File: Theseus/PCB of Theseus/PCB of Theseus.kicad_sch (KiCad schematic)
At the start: 47 parts, among them J1 Screw_Terminal_01x04, J2 Screw_Terminal_01x04, J4 Screw_Terminal_01x06, J7 Screw_Terminal_01x02, J8 Screw_Terminal_01x06, Q1 NMOS, Q2 NMOS, U1 TPS564257DRL, U2 MCP2562

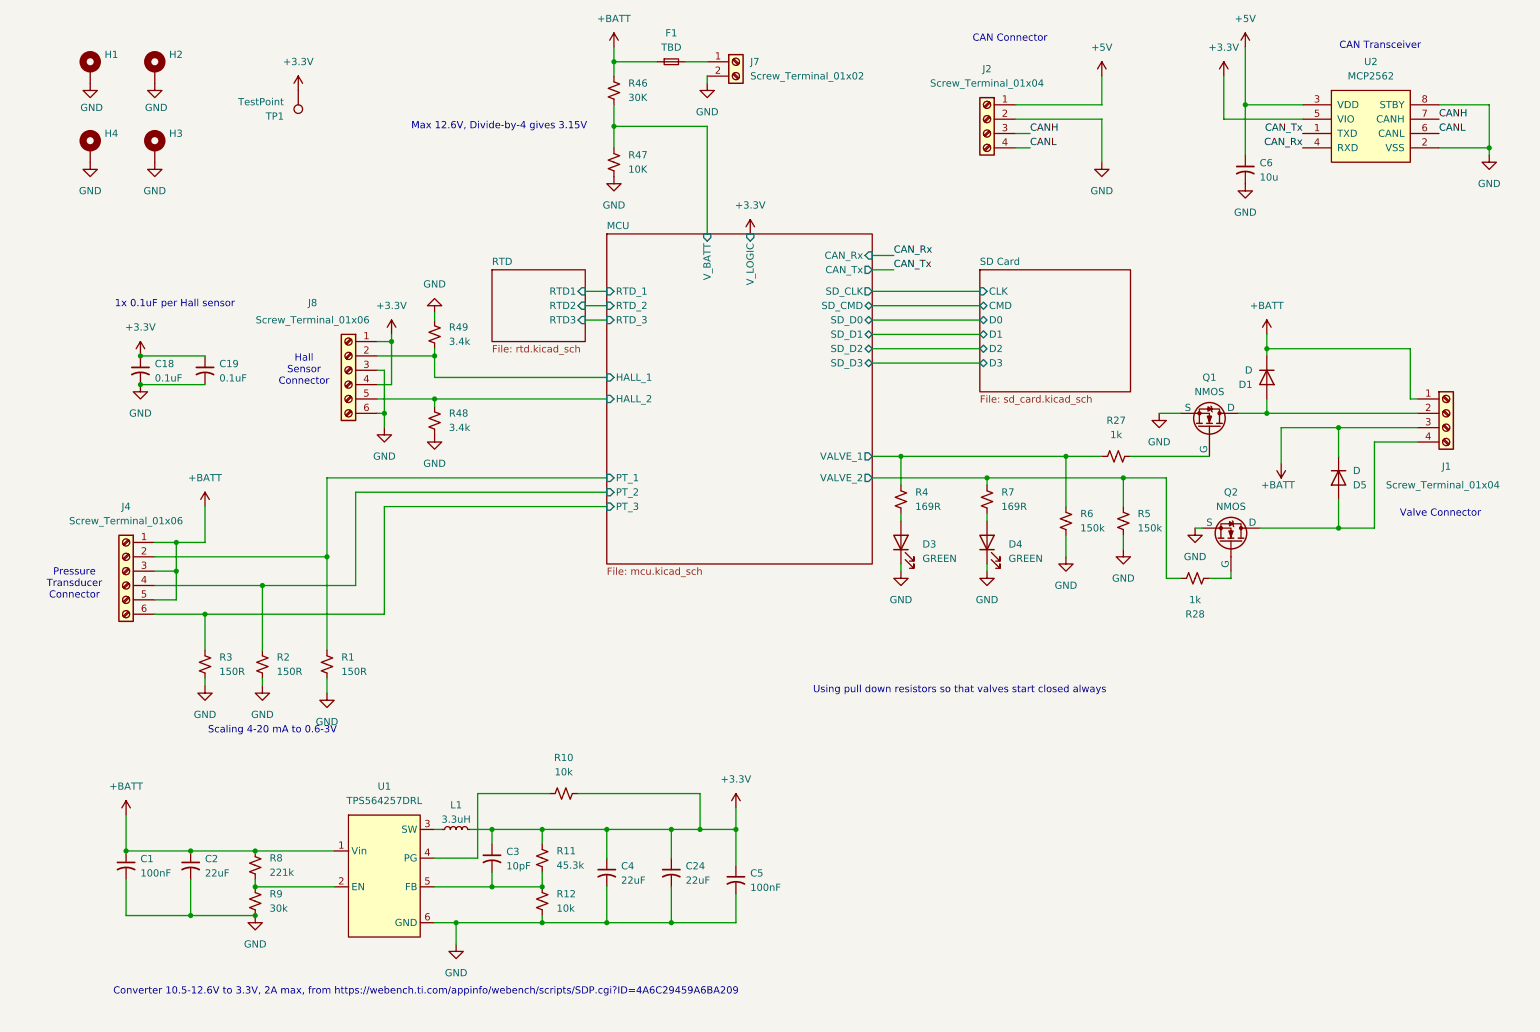
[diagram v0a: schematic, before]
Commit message: Theseus_Dev_Rev2
It's still the same PCB
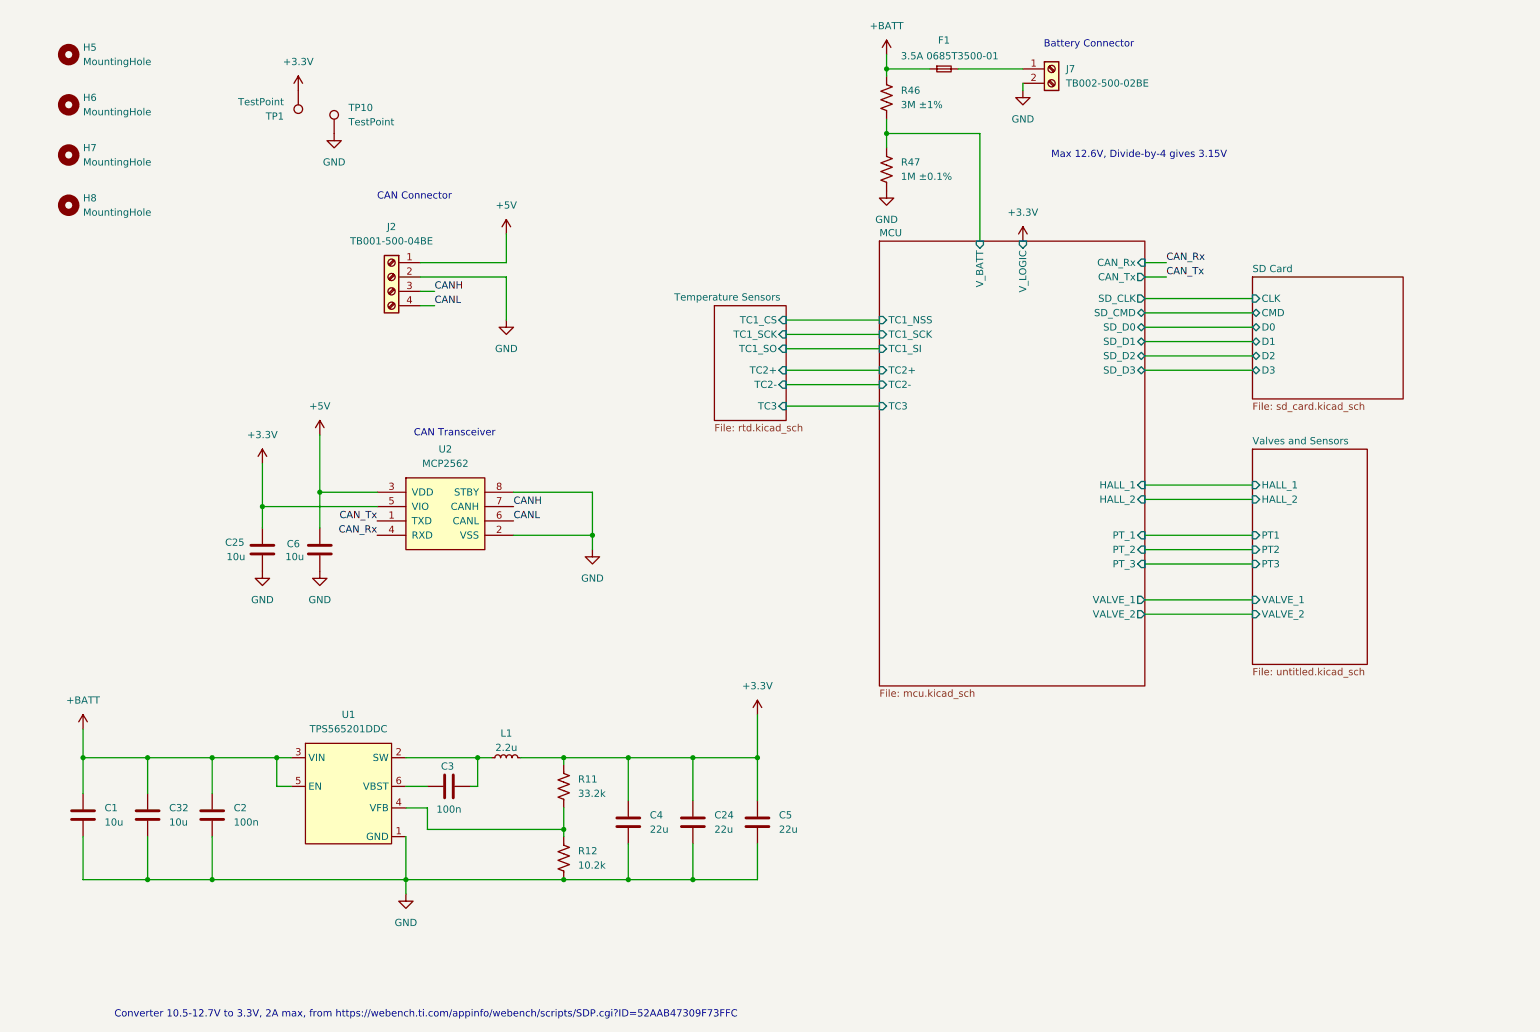
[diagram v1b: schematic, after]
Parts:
- removed C1, C5: 100nF, Capacitor_SMD:C_0603_1608Metric_Pad1.08x0.95mm_HandSolder, symbol Device:C_Small_US
- removed C18, C19: 0.1uF, Capacitor_SMD:C_0201_0603Metric_Pad0.64x0.40mm_HandSolder, symbol Device:C_Small_US
- removed C2, C24, C4: 22uF, Capacitor_SMD:C_0805_2012Metric_Pad1.18x1.45mm_HandSolder, symbol Device:C_Small_US
- removed C3: 10pF, Capacitor_SMD:C_0402_1005Metric_Pad0.74x0.62mm_HandSolder, symbol Device:C_Small_US
- removed C6: 10u, Capacitor_SMD:C_0603_1608Metric_Pad1.08x0.95mm_HandSolder, symbol Device:C_Small_US
- removed D1, D5: D, Diode_SMD:D_SMB-SMC_Universal_Handsoldering, symbol Device:D
- removed D3, D4: GREEN, Diode_SMD:D_0603_1608Metric_Pad1.05x0.95mm_HandSolder, symbol Device:LED
- removed H1, H2, H3, H4: ~, MountingHole:MountingHole_3.2mm_M3_Pad_Via, symbol Mechanical:MountingHole_Pad
- removed J1: Screw_Terminal_01x04, TerminalBlock_CUI:TerminalBlock_CUI_TB007-508-04_1x04_P5.08mm_Horizontal, symbol Connector:Screw_Terminal_01x04
- removed J4, J8: Screw_Terminal_01x06, TerminalBlock_CUI:TerminalBlock_CUI_TB007-508-06_1x06_P5.08mm_Horizontal, symbol Connector:Screw_Terminal_01x06
- removed Q1, Q2: NMOS, Package_TO_SOT_SMD:SOT-23-3, symbol Simulation_SPICE:NMOS
- removed R1, R2, R3: 150R, Resistor_SMD:R_0603_1608Metric_Pad0.98x0.95mm_HandSolder, symbol Device:R_Small_US
- removed R10: 10k, Resistor_SMD:R_0402_1005Metric_Pad0.72x0.64mm_HandSolder, symbol Device:R_Small_US
- removed R27, R28: 1k, Resistor_SMD:R_0402_1005Metric_Pad0.72x0.64mm_HandSolder, symbol Device:R_Small_US
- removed R4, R7: 169R, Resistor_SMD:R_0603_1608Metric_Pad0.98x0.95mm_HandSolder, symbol Device:R_Small_US
- removed R48, R49: 3.4k, Resistor_SMD:R_0402_1005Metric_Pad0.72x0.64mm_HandSolder, symbol Device:R_Small_US
- removed R5, R6: 150k, Resistor_SMD:R_0603_1608Metric_Pad0.98x0.95mm_HandSolder, symbol Device:R_Small_US
- removed R8: 221k, Resistor_SMD:R_0603_1608Metric_Pad0.98x0.95mm_HandSolder, symbol Device:R_Small_US
- removed R9: 30k, Resistor_SMD:R_0603_1608Metric_Pad0.98x0.95mm_HandSolder, symbol Device:R_Small_US
- removed U1: TPS564257DRL, Package_TO_SOT_SMD:SOT-563, symbol FYDP_Library:TPS564257DRL
- added C1, C25, C32, C6: 10u, Capacitor_SMD:C_0805_2012Metric_Pad1.18x1.45mm_HandSolder, symbol Device:C
- added C2, C3: 100n, Capacitor_SMD:C_0805_2012Metric_Pad1.18x1.45mm_HandSolder, symbol Device:C
- added C24, C4, C5: 22u, Capacitor_SMD:C_0805_2012Metric_Pad1.18x1.45mm_HandSolder, symbol Device:C
- added H5, H6, H7, H8: MountingHole, MountingHole:MountingHole_4.3mm_M4, symbol Mechanical:MountingHole
- added TP10: TestPoint, TestPoint:TestPoint_Pad_D2.0mm, symbol Connector:TestPoint
- added U1: TPS565201DDC, Package_TO_SOT_SMD:SOT-23-6_Handsoldering, symbol FYDP_Library:TPS565201DDC
- F1: value TBD -> 3.5A 0685T3500-01
- J2: value Screw_Terminal_01x04 -> TB001-500-04BE
- J7: value Screw_Terminal_01x02 -> TB002-500-02BE
- L1: value 3.3uH -> 2.2u; footprint Fydp_footprints:VLS6045EX-3R3N -> Fydp_footprints:SPM6530T-2R2M
- R11: value 45.3k -> 33.2k; footprint Resistor_SMD:R_0603_1608Metric_Pad0.98x0.95mm_HandSolder -> Resistor_SMD:R_0805_2012Metric_Pad1.20x1.40mm_HandSolder; symbol Device:R_Small_US -> Device:R_US
- R12: value 10k -> 10.2k; footprint Resistor_SMD:R_0402_1005Metric_Pad0.72x0.64mm_HandSolder -> Resistor_SMD:R_0805_2012Metric_Pad1.20x1.40mm_HandSolder; symbol Device:R_Small_US -> Device:R_US
- R46: value 30K -> 3M ±1%; footprint Resistor_SMD:R_0603_1608Metric_Pad0.98x0.95mm_HandSolder -> Resistor_SMD:R_0805_2012Metric_Pad1.20x1.40mm_HandSolder; symbol Device:R_Small_US -> Device:R_US
- R47: value 10K -> 1M ±0.1%; footprint Resistor_SMD:R_0402_1005Metric_Pad0.72x0.64mm_HandSolder -> Resistor_SMD:R_0805_2012Metric_Pad1.20x1.40mm_HandSolder; symbol Device:R_Small_US -> Device:R_US
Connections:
- net +3.3V: now also C24.1, C25.1, C4.1, C5.1
- net +5V: now also C6.1
- net +BATT: now also C1.1, C2.1, C32.1, U1.3 (VIN), U1.5 (EN)
- net GND: now also C1.2, C2.2, C24.2, C25.2, C32.2, C4.2, C5.2, C6.2, TP10.1, U1.1 (GND)
- net at L1.2: now also C3.1, U1.2 (SW)
- net at R11.2, R12.1: now also U1.4 (VFB)
- new net: C3.2, U1.6 (VBST)
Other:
- sheet RTD renamed Temperature Sensors
- added sheet Valves and Sensors (untitled.kicad_sch)
- sheet MCU ports: added TC1_NSS, TC1_SCK, TC1_SI, TC2+, TC2-, TC3; removed RTD_1, RTD_2, RTD_3
- sheet Temperature Sensors ports: added TC1_CS, TC1_SCK, TC1_SO, TC2+, TC2-, TC3; removed RTD1, RTD2, RTD3
- note added: "Battery Connector"
- note added: "Converter 10.5-12.7V to 3.3V, 2A max, from https://webench.ti.com/appinfo/webench/scripts/SDP.cgi?ID=52AAB47309F73FFC"
- note removed: "1x 0.1uF per Hall sensor"
- note removed: "Converter 10.5-12.6V to 3.3V, 2A max, from https://webench.ti.com/appinfo/webench/scripts/SDP.cgi?ID=4A6C29459A6BA209"
- note removed: "Hall Sensor Connector"
- note removed: "Pressure Transducer Connector"
- note removed: "Scaling 4-20 mA to 0.6-3V"
- note removed: "Using pull down resistors so that valves start closed always"
- note removed: "Valve Connector"
- moved on the sheet: F1, J2, J7, L1, U2
